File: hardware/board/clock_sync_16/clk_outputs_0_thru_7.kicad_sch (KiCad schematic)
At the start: 40 parts, among them J2 AudioJack3, U5 ISO6521FREUR

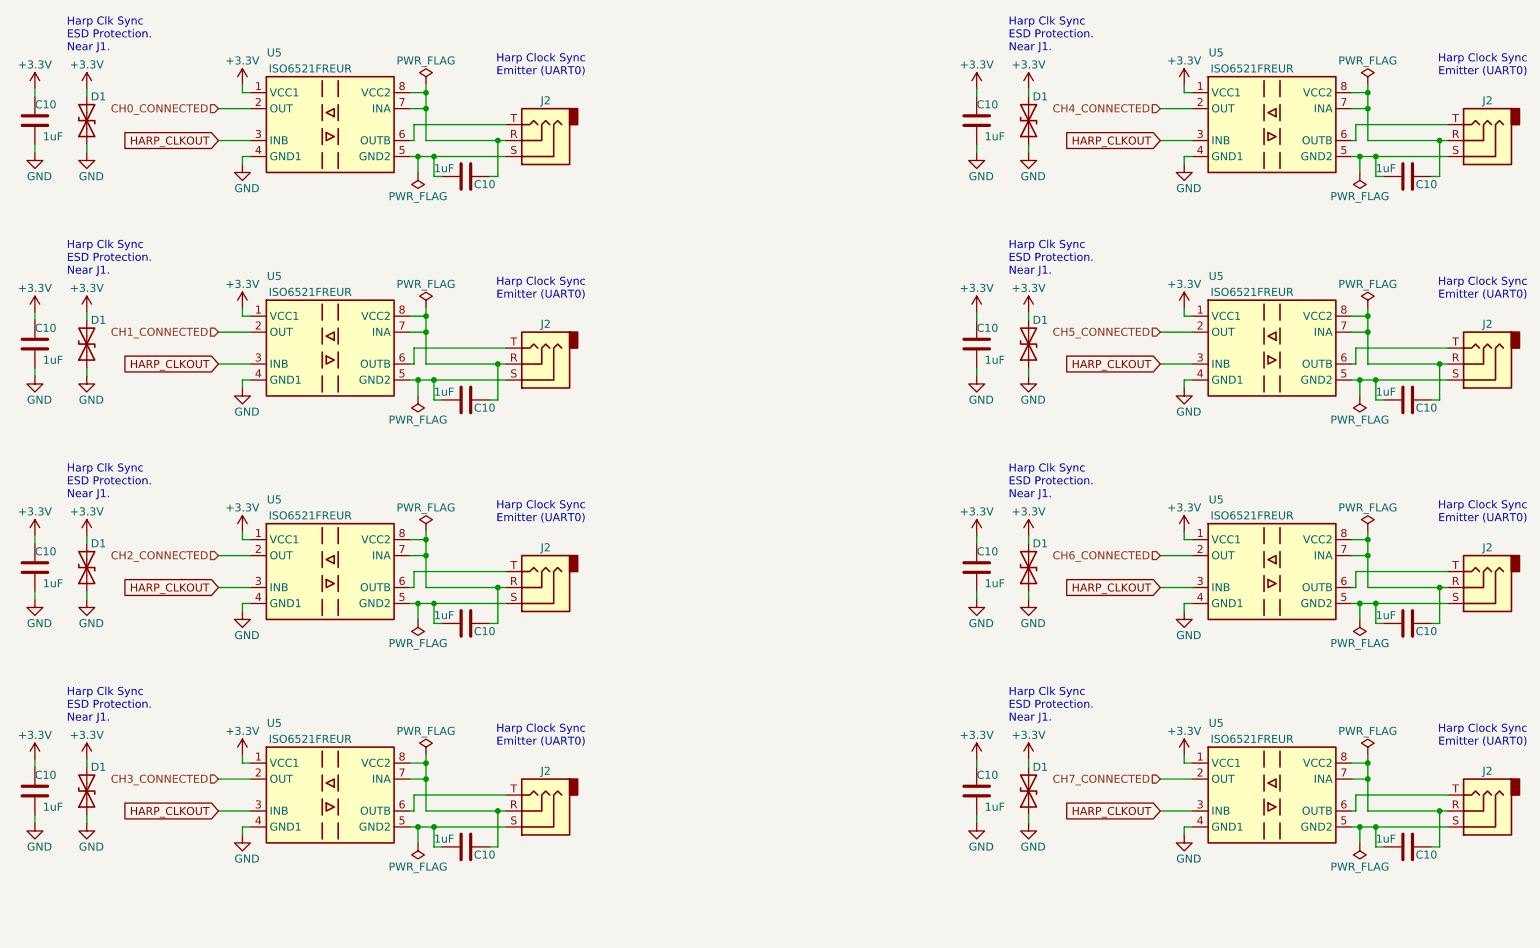
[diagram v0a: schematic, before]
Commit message: route pcb v0.1
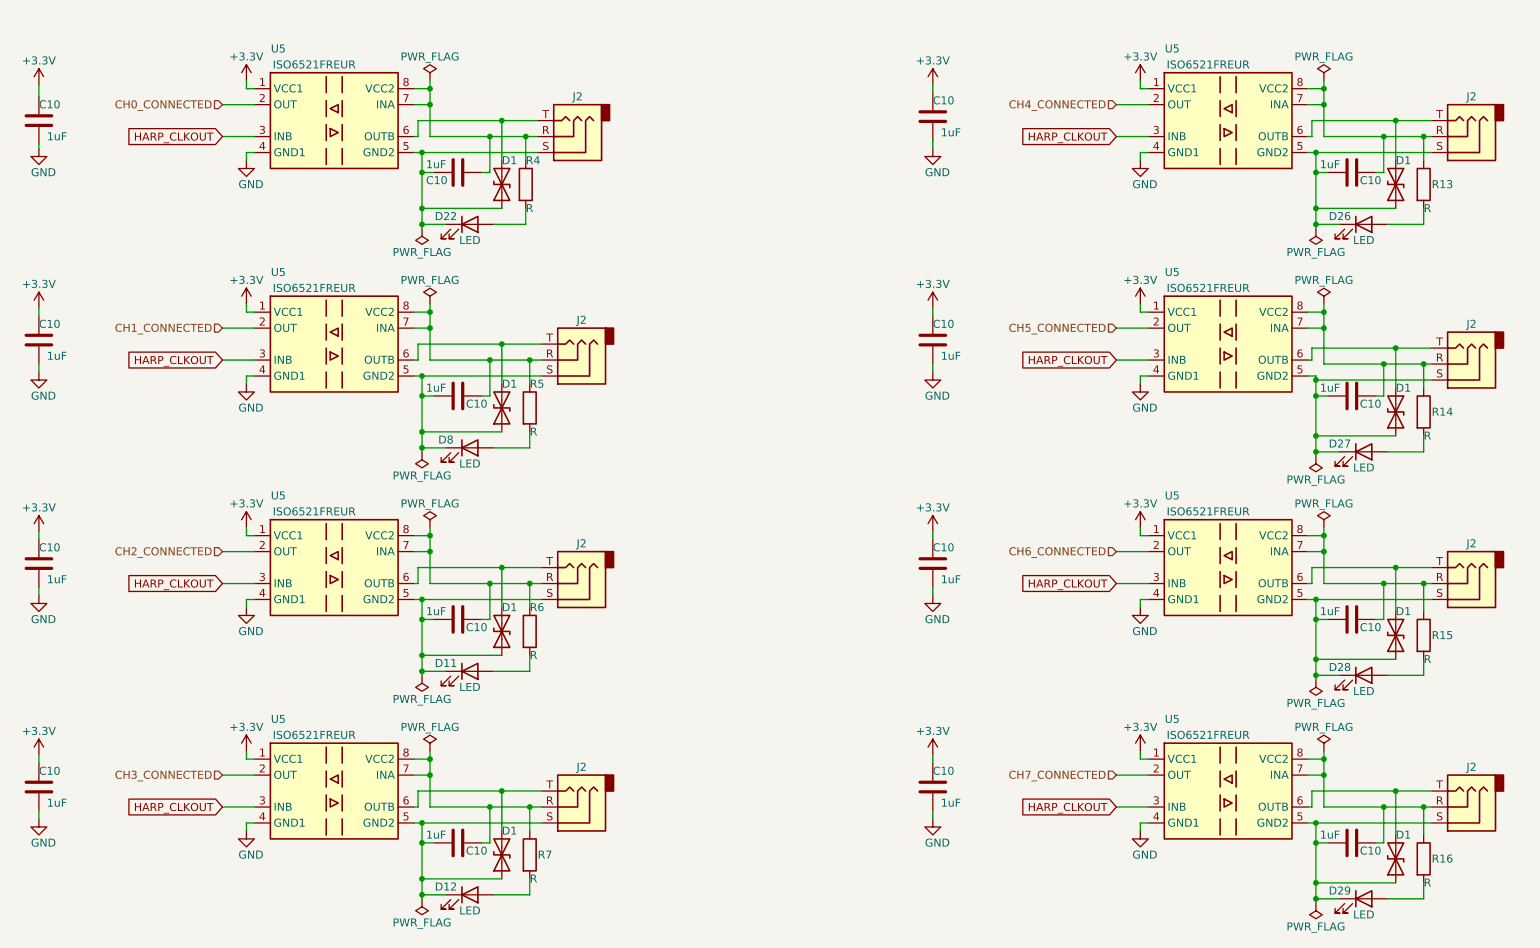
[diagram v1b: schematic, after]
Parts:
- removed C10 (x14): 1uF, Capacitor_SMD:C_0402_1005Metric, symbol Device:C
- removed D1 (x7): D_TVS, Diode_SMD:D_0402_1005Metric, symbol Device:D_TVS
- removed J2 (x7): AudioJack3, Connector_Audio:Jack_3.5mm_CUI_SJ-3523-SMT_Horizontal, symbol Connector:AudioJack3
- removed U5 (x7): ISO6521FREUR, kicad_component_library:DFN-8_3x2mm_P0.5mm, symbol kicad_component_library:ISO6521FREUR
- added C10 (x14): 1uF, Capacitor_SMD:C_0402_1005Metric, symbol Device:C
- added D1 (x7): D_TVS, Diode_SMD:D_0402_1005Metric, symbol Device:D_TVS
- added D11, D12, D22, D26, D27, D28, D29, D8: LED, LED_SMD:LED_0603_1608Metric_Pad1.05x0.95mm_HandSolder, symbol Device:LED
- added J2 (x7): AudioJack3, kicad_component_library:Jack_3.5mm_Kycon_STX-3680-5NB_Vertical, symbol Connector:AudioJack3
- added R13, R14, R15, R16, R4, R5, R6, R7: R, Resistor_SMD:R_0402_1005Metric, symbol Device:R
- added U5 (x7): ISO6521FREUR, kicad_component_library:DFN-8_3x2mm_P0.5mm, symbol kicad_component_library:ISO6521FREUR
- J2: footprint Connector_Audio:Jack_3.5mm_CUI_SJ-3523-SMT_Horizontal -> kicad_component_library:Jack_3.5mm_Kycon_STX-3680-5NB_Vertical; Link https://www.digikey.com/en/products/detail/cui-devices/SJ-3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 -> https://www.digikey.com/en/products/detail/kycon-inc/STX-36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; Manufacturer (none) -> Kycon; Manufacturer Number SJ-3523-SMT-TR -> STX-3680-5NB; PCBWay Link https://www.pcbway.com/components/detail/SJ3523SMTTR/473228/ -> (none)
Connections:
- net +3.3V: now also C10.1, C10.1, C10.1, C10.1, C10.1, C10.1, C10.1, C10.1, U5.1 (VCC1), U5.1 (VCC1), U5.1 (VCC1), U5.1 (VCC1), U5.1 (VCC1), U5.1 (VCC1), U5.1 (VCC1)
- net CH1_CONNECTED: now also U5.2 (OUT)
- net CH2_CONNECTED: now also U5.2 (OUT)
- net CH3_CONNECTED: now also U5.2 (OUT)
- net CH4_CONNECTED: now also U5.2 (OUT)
- net CH5_CONNECTED: now also U5.2 (OUT)
- net CH6_CONNECTED: now also U5.2 (OUT)
- net CH7_CONNECTED: now also U5.2 (OUT)
- net GND: now also C10.2, C10.2, C10.2, C10.2, C10.2, C10.2, C10.2, U5.4 (GND1), U5.4 (GND1), U5.4 (GND1), U5.4 (GND1), U5.4 (GND1), U5.4 (GND1), U5.4 (GND1); no longer D1.1 (A1)
- net HARP_CLKOUT: now also U5.3 (INB), U5.3 (INB), U5.3 (INB), U5.3 (INB), U5.3 (INB), U5.3 (INB), U5.3 (INB)
- net at C10.1, J2.R, U5.7 (INA)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: now also R4.1
- net at C10.2, J2.S, U5.5 (GND2): now also D1.1 (A1), D22.1 (K)
- net at J2.T, U5.6 (OUTB): now also D1.2 (A2)
- removed net +3V3: C10.1, D1.2 (A2)
- new net: C10.1, J2.R, R13.1, U5.7 (INA), U5.8 (VCC2)
- new net: D26.2 (A), R13.2
- new net: C10.2, D1.1 (A1), D8.1 (K), J2.S, U5.5 (GND2)
- new net: D1.2 (A2), J2.T, U5.6 (OUTB) (x7)
- new net: C10.1, J2.R, R5.1, U5.7 (INA), U5.8 (VCC2)
- new net: C10.2, D1.1 (A1), D12.1 (K), J2.S, U5.5 (GND2)
- new net: D12.2 (A), R7.2
- new net: C10.1, J2.R, R15.1, U5.7 (INA), U5.8 (VCC2)
- new net: C10.2, D1.1 (A1), D28.1 (K), J2.S, U5.5 (GND2)
- new net: C10.1, J2.R, R14.1, U5.7 (INA), U5.8 (VCC2)
- new net: C10.2, D1.1 (A1), D27.1 (K), J2.S, U5.5 (GND2)
- new net: C10.1, J2.R, R16.1, U5.7 (INA), U5.8 (VCC2)
- new net: C10.2, D1.1 (A1), D29.1 (K), J2.S, U5.5 (GND2)
- new net: C10.1, J2.R, R7.1, U5.7 (INA), U5.8 (VCC2)
- new net: D29.2 (A), R16.2
- new net: D27.2 (A), R14.2
- new net: C10.1, J2.R, R6.1, U5.7 (INA), U5.8 (VCC2)
- new net: C10.2, D1.1 (A1), D11.1 (K), J2.S, U5.5 (GND2)
- new net: D22.2 (A), R4.2
- new net: D28.2 (A), R15.2
- new net: C10.2, D1.1 (A1), D26.1 (K), J2.S, U5.5 (GND2)
- new net: D8.2 (A), R5.2
- new net: D11.2 (A), R6.2
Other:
- note removed: "Harp Clk Sync ESD Protection. Near J1."
- note removed: "Harp Clock Sync Emitter (UART0)"
- moved on the sheet: C10, D1, J2, U5
